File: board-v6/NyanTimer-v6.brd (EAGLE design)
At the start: 136.3 x 45 mm, 46 parts, among them IC1 7815DT, IC2 MAX232, IC3 7815DT, SW1 AKIZUKI_SWITCH, U1 328P

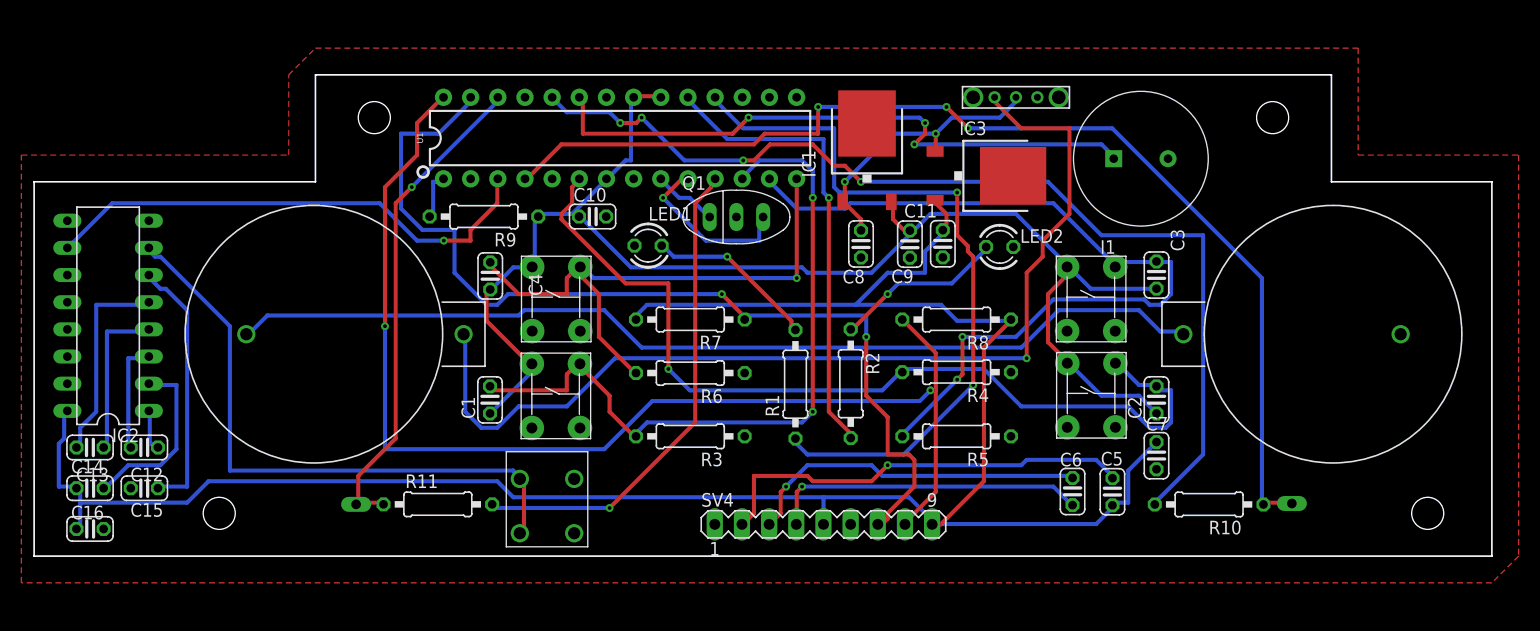
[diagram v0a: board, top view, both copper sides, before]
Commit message: modified board
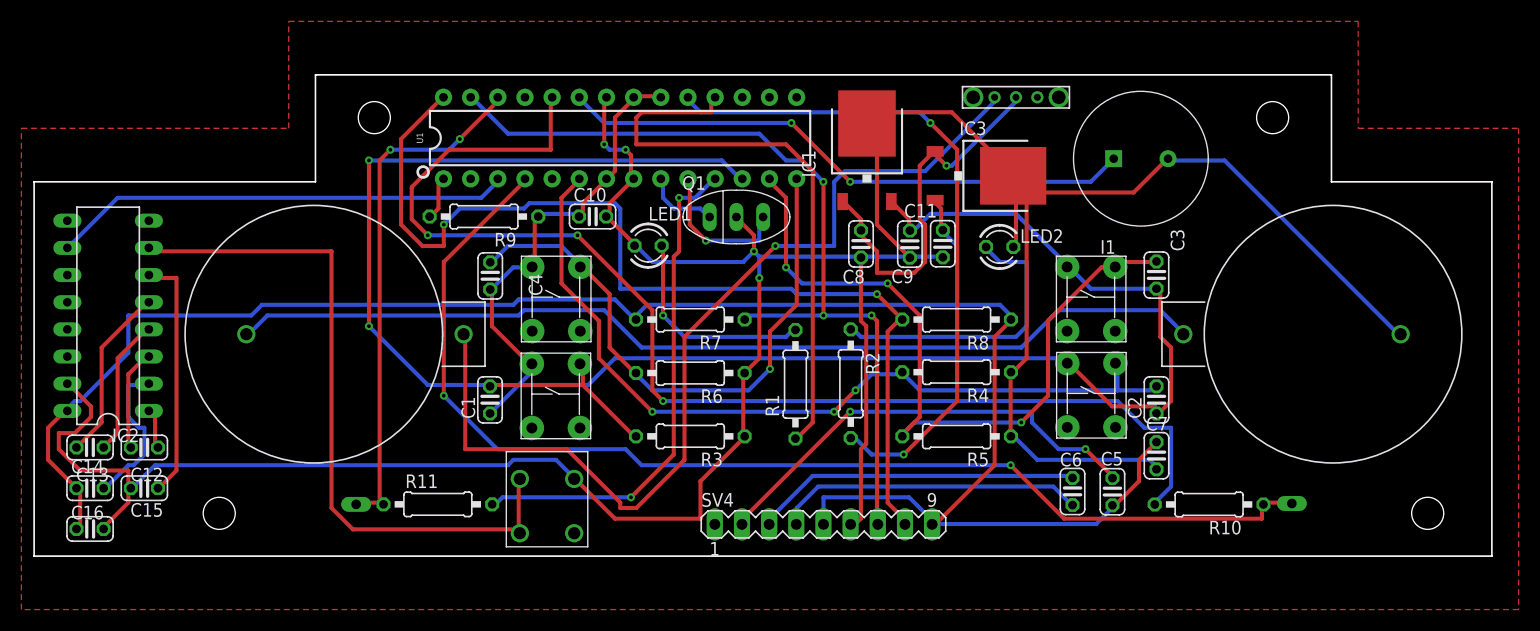
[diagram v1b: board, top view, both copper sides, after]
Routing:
- net GND: track 0.00 -> 309.2 mm, vias 0 -> 4
- net LEDG: track 43.4 -> 63.4 mm, vias 1 -> 2
- net PADRIN: track 94.9 -> 113.6 mm, vias 4 -> 3
- net +5V: track 132.7 -> 151.0 mm
- net SCL: track 110.8 -> 93.5 mm
- net VCC: track 199.9 -> 182.7 mm
- net SW1: track 67.7 -> 82.4 mm
- net LEDR: track 68.4 -> 54.5 mm, vias 2 -> 0
- net N$2: track 15.9 -> 27.5 mm, vias 1 -> 0
- net SDA: track 90.6 -> 80.6 mm, vias 2 -> 3
- net VSWOUT: track 26.5 -> 35.2 mm, vias 2 -> 1
- net SW3: track 78.0 -> 70.0 mm, vias 2 -> 3
- net PHONE: track 57.2 -> 64.8 mm
- net SW2: track 85.4 -> 78.3 mm, vias 1 -> 3
- net VSW: track 94.7 -> 89.3 mm
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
